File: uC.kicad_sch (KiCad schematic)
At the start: 6 parts, among them J2 OLED

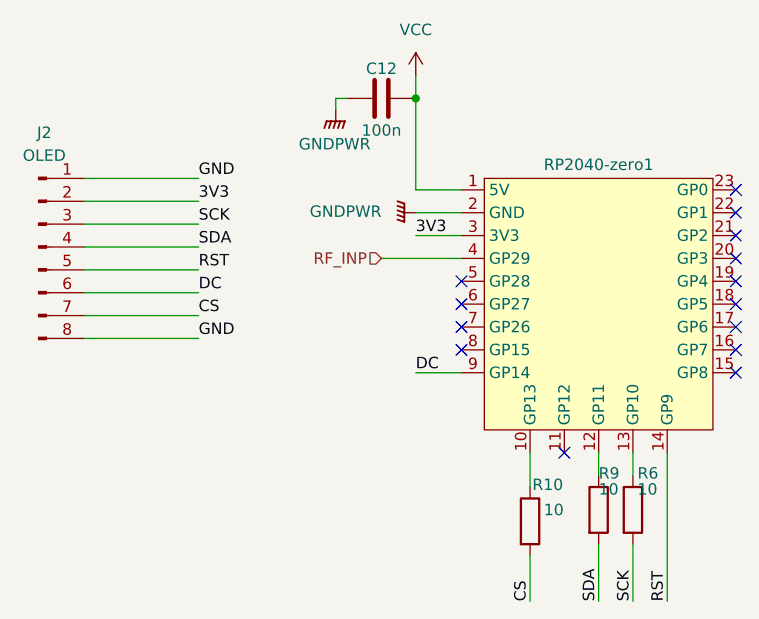
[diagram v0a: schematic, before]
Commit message: test2
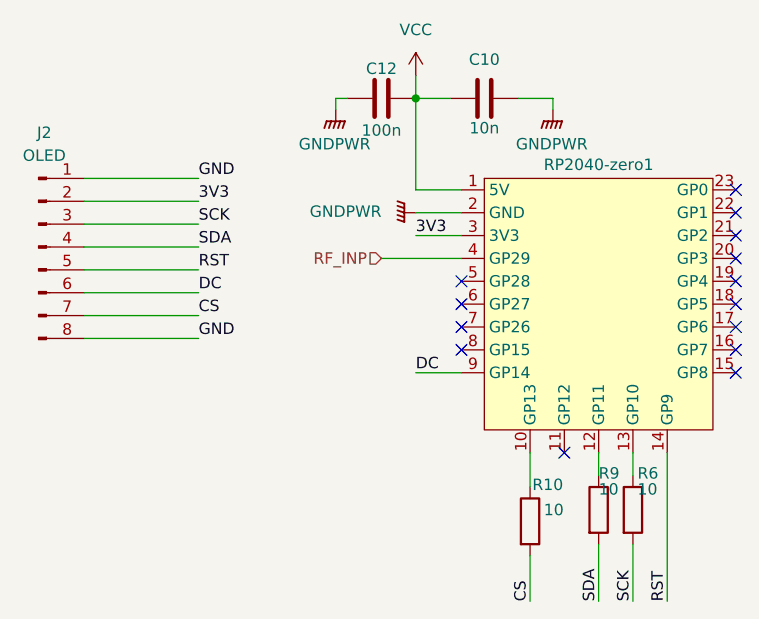
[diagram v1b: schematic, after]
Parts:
- added C10: 10n, Capacitor_SMD:C_1206_3216Metric_Pad1.33x1.80mm_HandSolder, symbol Device:C
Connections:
- net GNDPWR: now also C10.2
- net VCC: now also C10.1
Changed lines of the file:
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@@
+	(wire
+		(pts
+			(xy 90.17 35.56) (xy 93.98 35.56)
+		)
+		(stroke
+			(width 0)
+			(type default)
+		)
+	)
 	(wire
 		(pts
@@
 	(wire
 		(pts
+			(xy 101.6 35.56) (xy 105.41 35.56)
+		)
+		(stroke
+			(width 0)
+			(type default)
+		)
+	)
+	(wire
+		(pts
 			(xy 90.17 33.02) (xy 90.17 35.56)
 		)
@@
 		(pts
 			(xy 53.34 52.07) (xy 66.04 52.07)
+		)
+		(stroke
+			(width 0)
+			(type default)
+		)
+	)
+	(wire
+		(pts
+			(xy 105.41 35.56) (xy 105.41 36.83)
 		)
 		(stroke
@@
 		)
 	)
+	(symbol
+		(lib_id "Device:C")
+		(at 97.79 35.56 90)
+		(unit 1)
+		(exclude_from_sim no)
+		(in_bom yes)
+		(on_board yes)
+		(dnp no)
+		(property "Reference" "C10"
+			(at 97.79 31.242 90)
+			(effects
+				(font
+					(size 1.27 1.27)
+				)
+			)
+		)
+		(property "Value" "10n"
+			(at 97.79 38.862 90)
+			(effects
+				(font
+					(size 1.27 1.27)
+				)
+			)
+		)
+		(property "Footprint" "Capacitor_SMD:C_1206_3216Metric_Pad1.33x1.80mm_HandSolder"
+			(at 101.6 34.5948 0)
+			(effects
+				(font
+					(size 1.27 1.27)
+				)
+				(hide yes)
+			)
+		)
+		(property "Datasheet" "~"
+			(at 97.79 35.56 0)
+			(effects
+				(font
+					(size 1.27 1.27)
+				)
+				(hide yes)
+			)
+		)
+		(property "Description" "Unpolarized capacitor"
+			(at 97.79 35.56 0)
+			(effects
+				(font
+					(size 1.27 1.27)
+				)
+				(hide yes)
+			)
+		)
+		(pin "2"
+		)
+		(pin "1"
+		)
+		(instances
+			(project ""
+				(path "/6e9b0ecb-5ff8-4cea-bb01-e8c92e636c95/47922e9f-8839-4dfe-b2ac-5d132f76ea44"
+					(reference "C10")
+					(unit 1)
+				)
+			)
+		)
+	)
+	(symbol
+		(lib_id "power:GNDPWR")
+		(at 105.41 36.83 0)
+		(unit 1)
+		(exclude_from_sim no)
+		(in_bom yes)
+		(on_board yes)
+		(dnp no)
+		(fields_autoplaced yes)
+		(property "Reference" "#PWR025"
+			(at 105.41 41.91 0)
+			(effects
+				(font
+					(size 1.27 1.27)
+				)
+				(hide yes)
+			)
+		)
+		(property "Value" "GNDPWR"
+			(at 105.283 40.64 0)
+			(effects
+				(font
+					(size 1.27 1.27)
+				)
+			)
+		)
+		(property "Footprint" ""
+			(at 105.41 38.1 0)
+			(effects
+				(font
+					(size 1.27 1.27)
+				)
+				(hide yes)
+			)
+		)
+		(property "Datasheet" ""
+			(at 105.41 38.1 0)
+			(effects
+				(font
+					(size 1.27 1.27)
+				)
+				(hide yes)
+			)
+		)
+		(property "Description" "Power symbol creates a global label with name \"GNDPWR\" , global ground"
+			(at 105.41 36.83 0)
+			(effects
+				(font
+					(size 1.27 1.27)
+				)
+				(hide yes)
+			)
+		)
+		(pin "1"
+		)
+		(instances
+			(project ""
+				(path "/6e9b0ecb-5ff8-4cea-bb01-e8c92e636c95/47922e9f-8839-4dfe-b2ac-5d132f76ea44"
+					(reference "#PWR025")
+					(unit 1)
+				)
+			)
+		)
+	)

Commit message: Kondensator usunięty Test2
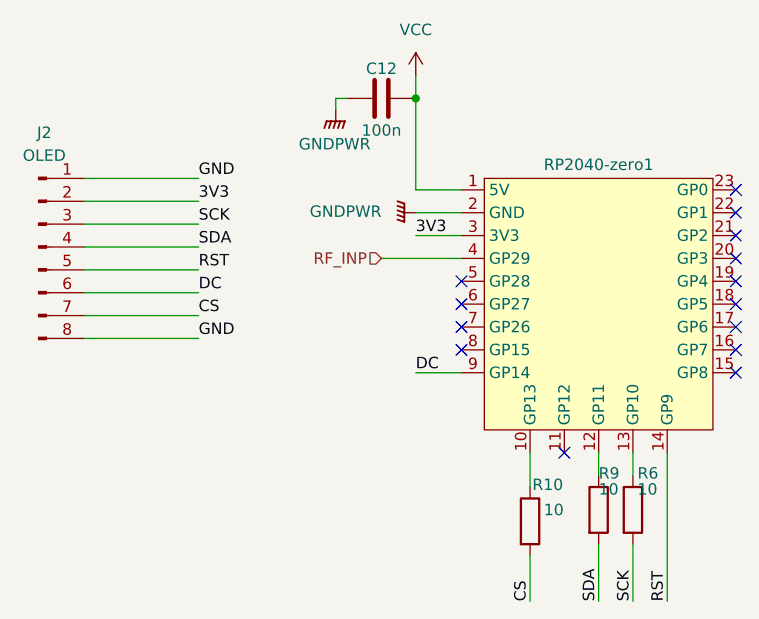
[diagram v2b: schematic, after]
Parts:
- removed C10: 10n, Capacitor_SMD:C_1206_3216Metric_Pad1.33x1.80mm_HandSolder, symbol Device:C
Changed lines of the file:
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@@
-	(wire
-		(pts
-			(xy 90.17 35.56) (xy 93.98 35.56)
-		)
-		(stroke
-			(width 0)
-			(type default)
-		)
-	)
 	(wire
 		(pts
@@
 	(wire
 		(pts
-			(xy 101.6 35.56) (xy 105.41 35.56)
-		)
-		(stroke
-			(width 0)
-			(type default)
-		)
-	)
-	(wire
-		(pts
 			(xy 90.17 33.02) (xy 90.17 35.56)
 		)
@@
 		(pts
 			(xy 53.34 52.07) (xy 66.04 52.07)
-		)
-		(stroke
-			(width 0)
-			(type default)
-		)
-	)
-	(wire
-		(pts
-			(xy 105.41 35.56) (xy 105.41 36.83)
 		)
 		(stroke
@@
 		)
 	)
-	(symbol
-		(lib_id "Device:C")
-		(at 97.79 35.56 90)
-		(unit 1)
-		(exclude_from_sim no)
-		(in_bom yes)
-		(on_board yes)
-		(dnp no)
-		(property "Reference" "C10"
-			(at 97.79 31.242 90)
-			(effects
-				(font
-					(size 1.27 1.27)
-				)
-			)
-		)
-		(property "Value" "10n"
-			(at 97.79 38.862 90)
-			(effects
-				(font
-					(size 1.27 1.27)
-				)
-			)
-		)
-		(property "Footprint" "Capacitor_SMD:C_1206_3216Metric_Pad1.33x1.80mm_HandSolder"
-			(at 101.6 34.5948 0)
-			(effects
-				(font
-					(size 1.27 1.27)
-				)
-				(hide yes)
-			)
-		)
-		(property "Datasheet" "~"
-			(at 97.79 35.56 0)
-			(effects
-				(font
-					(size 1.27 1.27)
-				)
-				(hide yes)
-			)
-		)
-		(property "Description" "Unpolarized capacitor"
-			(at 97.79 35.56 0)
-			(effects
-				(font
-					(size 1.27 1.27)
-				)
-				(hide yes)
-			)
-		)
-		(pin "2"
-		)
-		(pin "1"
-		)
-		(instances
-			(project ""
-				(path "/6e9b0ecb-5ff8-4cea-bb01-e8c92e636c95/47922e9f-8839-4dfe-b2ac-5d132f76ea44"
-					(reference "C10")
-					(unit 1)
-				)
-			)
-		)
-	)
-	(symbol
-		(lib_id "power:GNDPWR")
-		(at 105.41 36.83 0)
-		(unit 1)
-		(exclude_from_sim no)
-		(in_bom yes)
-		(on_board yes)
-		(dnp no)
-		(fields_autoplaced yes)
-		(property "Reference" "#PWR025"
-			(at 105.41 41.91 0)
-			(effects
-				(font
-					(size 1.27 1.27)
-				)
-				(hide yes)
-			)
-		)
-		(property "Value" "GNDPWR"
-			(at 105.283 40.64 0)
-			(effects
-				(font
-					(size 1.27 1.27)
-				)
-			)
-		)
-		(property "Footprint" ""
-			(at 105.41 38.1 0)
-			(effects
-				(font
-					(size 1.27 1.27)
-				)
-				(hide yes)
-			)
-		)
-		(property "Datasheet" ""
-			(at 105.41 38.1 0)
-			(effects
-				(font
-					(size 1.27 1.27)
-				)
-				(hide yes)
-			)
-		)
-		(property "Description" "Power symbol creates a global label with name \"GNDPWR\" , global ground"
-			(at 105.41 36.83 0)
-			(effects
-				(font
-					(size 1.27 1.27)
-				)
-				(hide yes)
-			)
-		)
-		(pin "1"
-		)
-		(instances
-			(project ""
-				(path "/6e9b0ecb-5ff8-4cea-bb01-e8c92e636c95/47922e9f-8839-4dfe-b2ac-5d132f76ea44"
-					(reference "#PWR025")
-					(unit 1)
-				)
-			)
-		)
-	)
